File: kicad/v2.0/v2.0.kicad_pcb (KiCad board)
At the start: 2 copper layers, 54.1 x 99.1 mm, 34 parts, among them J1 9V_IN, J2 BUTTON, J3 LED STRIP, J4 MOTOR, J5 DEV BOARD LEFT, J6 DEV BOARD RIGHT, Q1 FQP30N06L, U1 L293D, U2 L7805

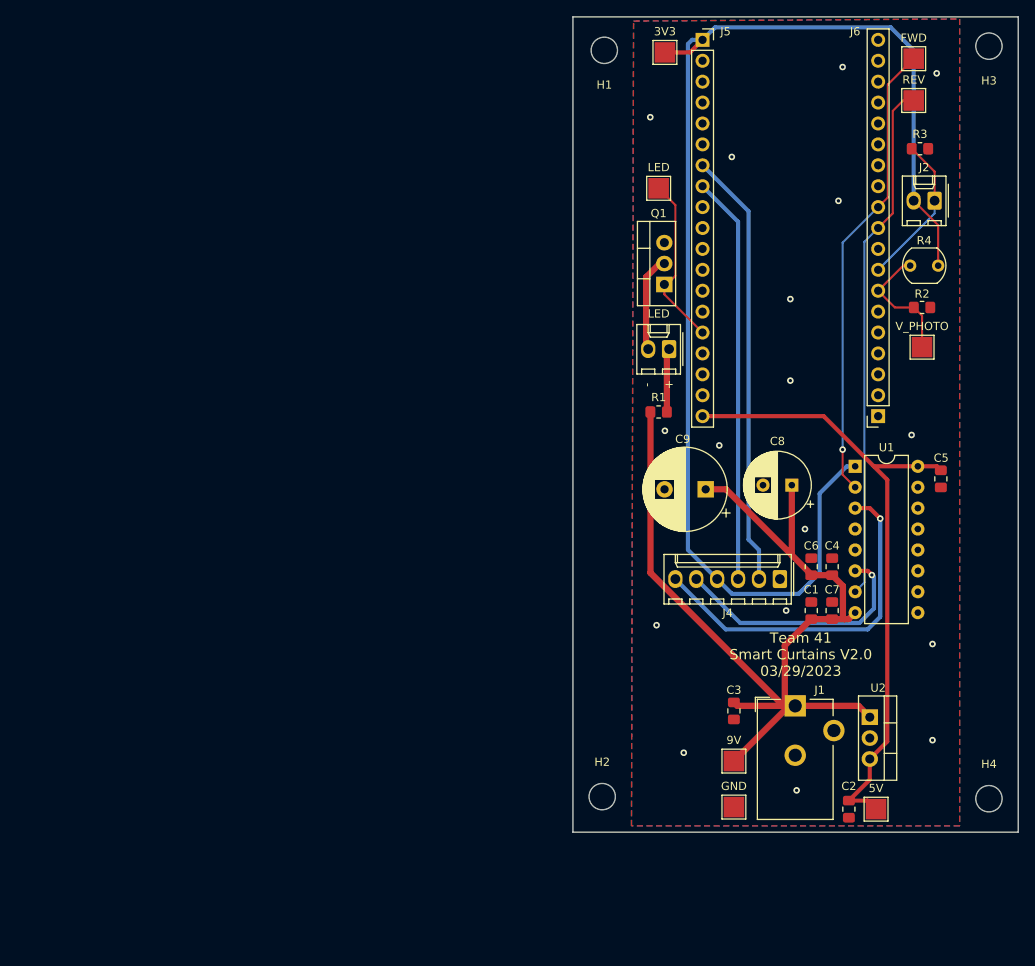
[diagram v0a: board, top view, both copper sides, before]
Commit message: minor changes to pcb
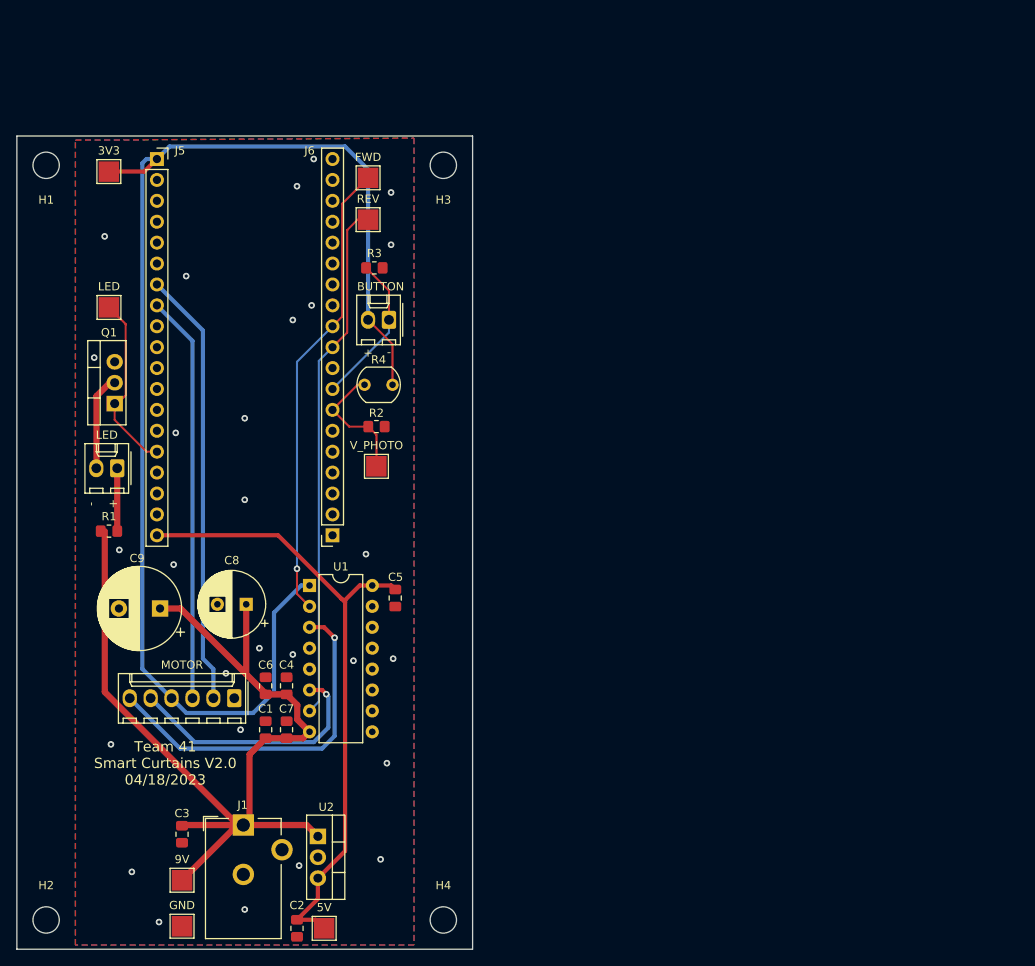
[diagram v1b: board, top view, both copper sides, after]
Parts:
- moved H1 69.2 mm to (124.2, 50.8)
- moved H2 69.2 mm to (124.2, 142.5)
- moved TP4 69.1 mm to (131.8, 51.6)
- moved C3 68.7 mm to (140.7, 132.1)
- moved J1 68.6 mm to (148.2, 131.0)
- moved TP3 68.6 mm to (158.0, 143.5)
- moved U2 68.6 mm to (157.2, 132.3)
- moved TP1 68.6 mm to (140.7, 143.3)
- moved TP2 68.6 mm to (140.7, 137.7)
- moved C2 68.6 mm to (154.7, 143.5)
- moved J3 68.6 mm to (132.8, 87.6)
- moved Q1 68.3 mm to (132.5, 79.8)
- moved R1 68.3 mm to (131.8, 95.2)
- moved TP7 68.3 mm to (131.8, 68.1)
- moved H4 67.9 mm to (172.5, 142.5)
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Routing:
- net +9V: track 123.1 -> 121.7 mm
- net +3V3: track 158.1 -> 159.4 mm
- net /LED: track 21.0 -> 22.0 mm
- net GND: vias 17 -> 29
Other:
- board size 54.1 x 99.1 mm -> 55.4 x 98.8 mm
- board text added: "Team 41 Smart Curtains V2.0 04/18/2023"
- board text removed: "Team 41 Smart Curtains V2.0 03/29/2023"
